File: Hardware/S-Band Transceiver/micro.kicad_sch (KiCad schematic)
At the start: 46 parts, among them J3 AVR-UPDI-6, J4 USB_C_Receptacle_USB2.0_16P, SW1 SW_Push, U2 AVR128DA48x-xPT, U3 ADS1118IDGS, U4 FT231XQ

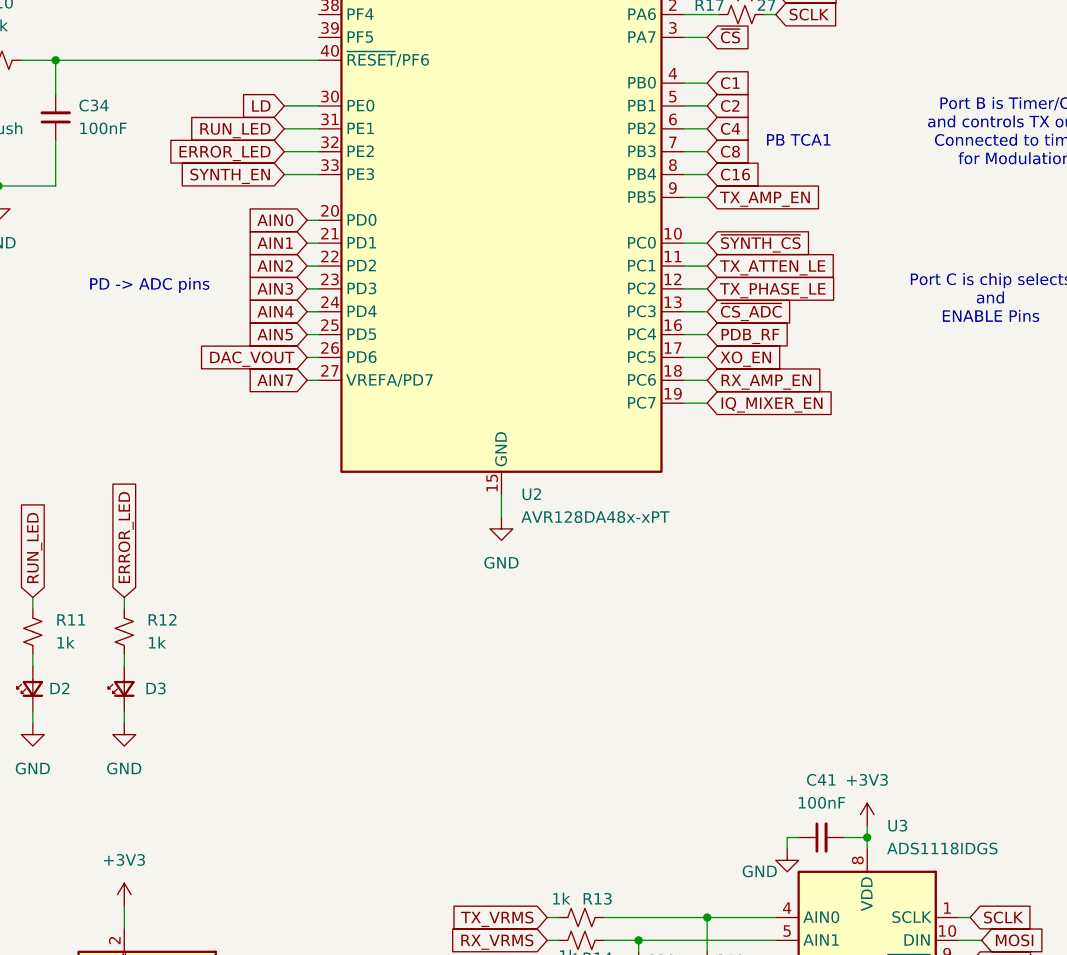
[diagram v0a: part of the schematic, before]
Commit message: Updating routing
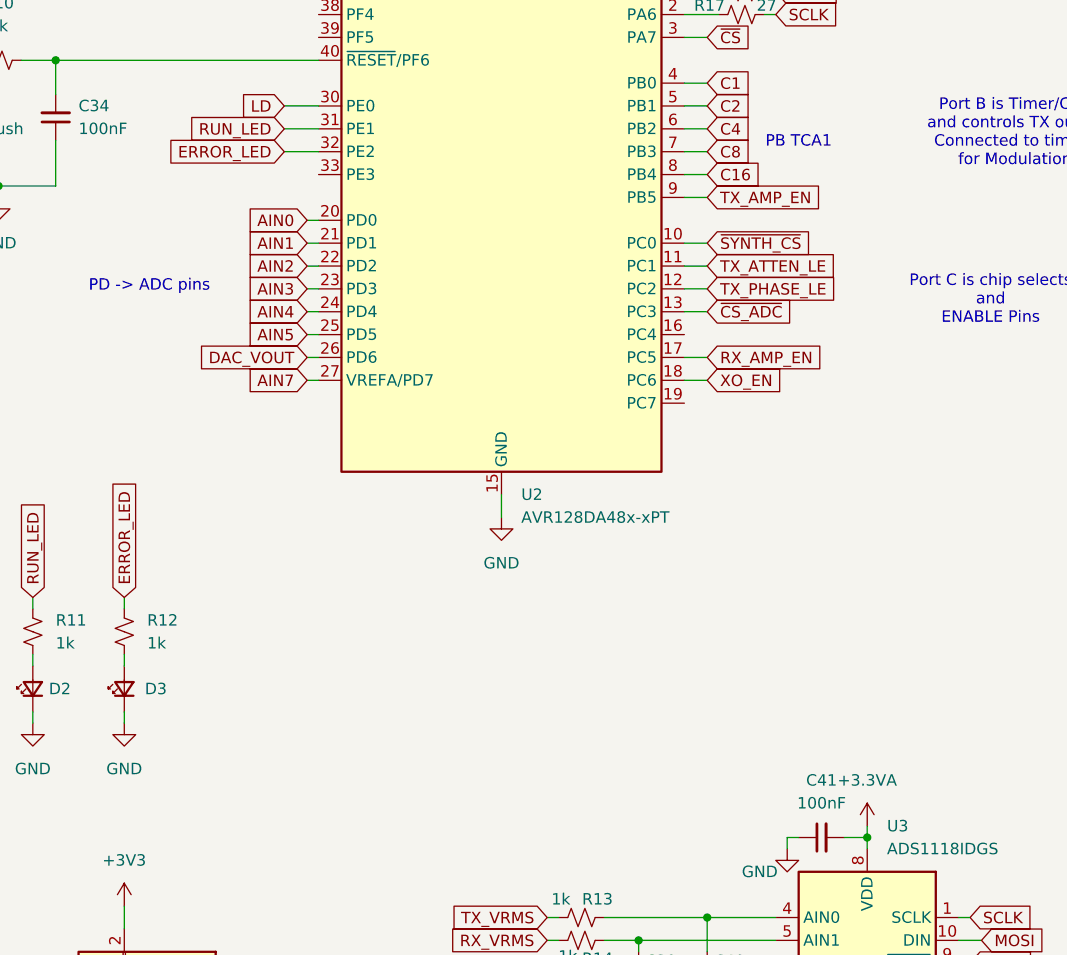
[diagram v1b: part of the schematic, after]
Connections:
- net +3V3: no longer C41.2, U3.8 (VDD)
- net RX_AMP_EN: now also U2.17 (PC5); no longer U2.18 (PC6)
- net XO_EN: now also U2.18 (PC6); no longer U2.17 (PC5)
- net IQ_MIXER_EN: no longer names the net of U2.19 (PC7)
- net PDB_RF: no longer names the net of U2.16 (PC4)
- net SYNTH_EN: no longer names the net of U2.33 (PE3)
- new net +3.3VA: C41.2, U3.8 (VDD)
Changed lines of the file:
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@@
 	(wire
 		(pts
-			(xy 100.33 96.52) (xy 102.87 96.52)
-		)
-		(stroke
-			(width 0)
-			(type default)
-		)
-	)
-	(wire
-		(pts
 			(xy 245.11 31.75) (xy 241.3 31.75)
 		)
@@
 	(wire
 		(pts
-			(xy 100.33 88.9) (xy 102.87 88.9)
-		)
-		(stroke
-			(width 0)
-			(type default)
-		)
-	)
-	(wire
-		(pts
 			(xy 187.96 120.65) (xy 203.2 120.65)
 		)
@@
 	(wire
 		(pts
-			(xy 55.88 71.12) (xy 59.69 71.12)
-		)
-		(stroke
-			(width 0)
-			(type default)
-		)
-	)
-	(wire
-		(pts
 			(xy 118.11 144.78) (xy 120.65 144.78)
 		)
@@
 		)
 	)
-	(global_label "PDB_RF"
-		(shape input)
-		(at 102.87 88.9 0)
-		(fields_autoplaced yes)
-		(effects
-			(font
-				(size 1.27 1.27)
-			)
-			(justify left)
-		)
-		(property "Intersheetrefs" "${INTERSHEET_REFS}"
-			(at 112.9914 88.9 0)
-			(effects
-				(font
-					(size 1.27 1.27)
-				)
-				(justify left)
-				(hide yes)
-			)
-		)
-	)
 	(global_label "AIN1"
 		(shape input)
@@
 		)
 	)
-	(global_label "SYNTH_EN"
-		(shape input)
-		(at 55.88 71.12 180)
-		(fields_autoplaced yes)
-		(effects
-			(font
-				(size 1.27 1.27)
-			)
-			(justify right)
-		)
-		(property "Intersheetrefs" "${INTERSHEET_REFS}"
-			(at 43.521 71.12 0)
-			(effects
-				(font
-					(size 1.27 1.27)
-				)
-				(justify right)
-				(hide yes)
-			)
-		)
-	)
 	(global_label "C8"
 		(shape input)
@@
 	(global_label "XO_EN"
 		(shape input)
-		(at 102.87 91.44 0)
+		(at 102.87 93.98 0)
 		(fields_autoplaced yes)
 		(effects
@@
 		)
 		(property "Intersheetrefs" "${INTERSHEET_REFS}"
-			(at 111.8423 91.44 0)
+			(at 111.8423 93.98 0)
 			(effects
 				(font
@@
 	(global_label "RX_AMP_EN"
 		(shape input)
-		(at 102.87 93.98 0)
+		(at 102.87 91.44 0)
 		(fields_autoplaced yes)
 		(effects
@@
 		)
 		(property "Intersheetrefs" "${INTERSHEET_REFS}"
-			(at 116.5594 93.98 0)
+			(at 116.5594 91.44 0)
 			(effects
 				(font
@@
 		)
 	)
-	(global_label "IQ_MIXER_EN"
-		(shape input)
-		(at 102.87 96.52 0)
-		(fields_autoplaced yes)
-		(effects
-			(font
-				(size 1.27 1.27)
-			)
-			(justify left)
-		)
-		(property "Intersheetrefs" "${INTERSHEET_REFS}"
-			(at 117.8899 96.52 0)
-			(effects
-				(font
-					(size 1.27 1.27)
-				)
-				(justify left)
-				(hide yes)
-			)
-		)
-	)
 	(global_label "DAC_VOUT"
 		(shape input)
@@
 	)
 	(symbol
+		(lib_id "power:+3.3VA")
+		(at 120.65 143.51 0)
+		(unit 1)
+		(exclude_from_sim no)
+		(in_bom yes)
+		(on_board yes)
+		(dnp no)
+		(fields_autoplaced yes)
+		(property "Reference" "#PWR043"
+			(at 120.65 147.32 0)
+			(effects
+				(font
+					(size 1.27 1.27)
+				)
+				(hide yes)
+			)
+		)
+		(property "Value" "+3.3VA"
+			(at 120.65 138.43 0)
+			(effects
+				(font
+					(size 1.27 1.27)
+				)
+			)
+		)
+		(property "Footprint" ""
+			(at 120.65 143.51 0)
+			(effects
+				(font
+					(size 1.27 1.27)
+				)
+				(hide yes)
+			)
+		)
+		(property "Datasheet" ""
+			(at 120.65 143.51 0)
+			(effects
+				(font
+					(size 1.27 1.27)
+				)
+				(hide yes)
+			)
+		)
+		(property "Description" "Power symbol creates a global label with name \"+3.3VA\""
+			(at 120.65 143.51 0)
+			(effects
+				(font
+					(size 1.27 1.27)
+				)
+				(hide yes)
+			)
+		)
+		(pin "1"
+		)
+		(instances
+			(project "S-Band Transceiver"
+				(path "/811f57cf-e3df-4fba-aff9-353adc85299e/03e3241c-59a9-4f6f-b7cc-ae3fa2c59abc"
+					(reference "#PWR043")
+					(unit 1)
+				)
+			)
+		)
+	)
+	(symbol
 		(lib_id "Device:R_Small_US")
 		(at 88.9 153.67 90)
@@
 					(unit 1)
 				)
-			)
-		)
-	)
-	(symbol
-		(lib_id "power:+3V3")
-		(at 120.65 143.51 0)
-		(unit 1)
-		(exclude_from_sim no)
-		(in_bom yes)
-		(on_board yes)
-		(dnp no)
-		(fields_autoplaced yes)
-		(property "Reference" "#PWR043"
-			(at 120.65 147.32 0)
-			(effects
-				(font
-					(size 1.27 1.27)
-				)
-				(hide yes)
-			)
-		)
-		(property "Value" "+3V3"
-			(at 120.65 138.43 0)
-			(effects
-				(font
-					(size 1.27 1.27)
-				)
-			)
-		)
-		(property "Footprint" ""
-			(at 120.65 143.51 0)
-			(effects
-				(font
-					(size 1.27 1.27)
-				)
-				(hide yes)
-			)
-		)
-		(property "Datasheet" ""
-			(at 120.65 143.51 0)
-			(effects
-				(font
-					(size 1.27 1.27)
-				)
-				(hide yes)
-			)
-		)
-		(property "Description" "Power symbol creates a global label with name \"+3V3\""
-			(at 120.65 143.51 0)
-			(effects
-				(font
-					(size 1.27 1.27)
-				)
-				(hide yes)
-			)
-		)
-		(pin "1"
-		)
-		(instances
-			(project "S-Band Transceiver"
-				(path "/811f57cf-e3df-4fba-aff9-353adc85299e/03e3241c-59a9-4f6f-b7cc-ae3fa2c59abc"
-					(reference "#PWR043")
-					(unit 1)
-				)
